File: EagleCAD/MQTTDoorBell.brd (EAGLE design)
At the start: 71.1 x 64.2 mm, 16 parts, among them Q1 MMBT2222

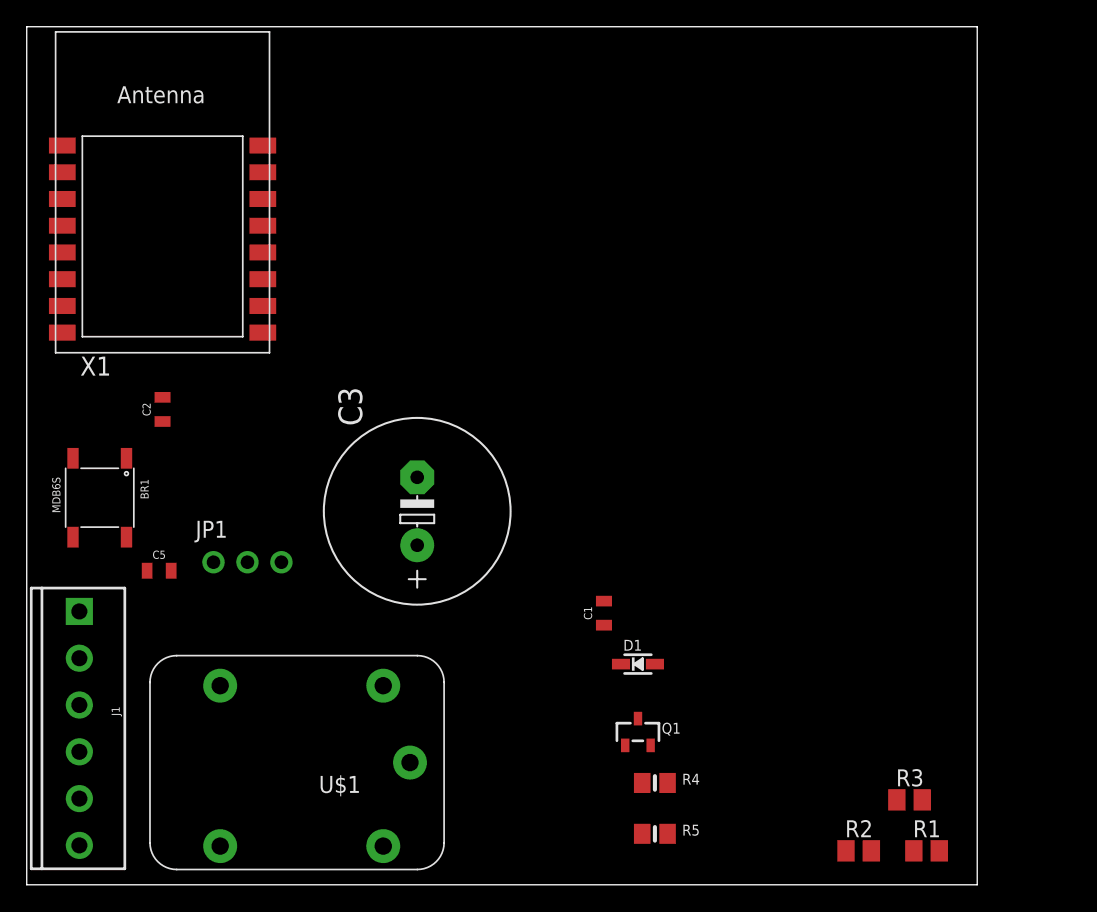
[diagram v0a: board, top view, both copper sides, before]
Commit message: initial commit of eagle files, version 1 of board'
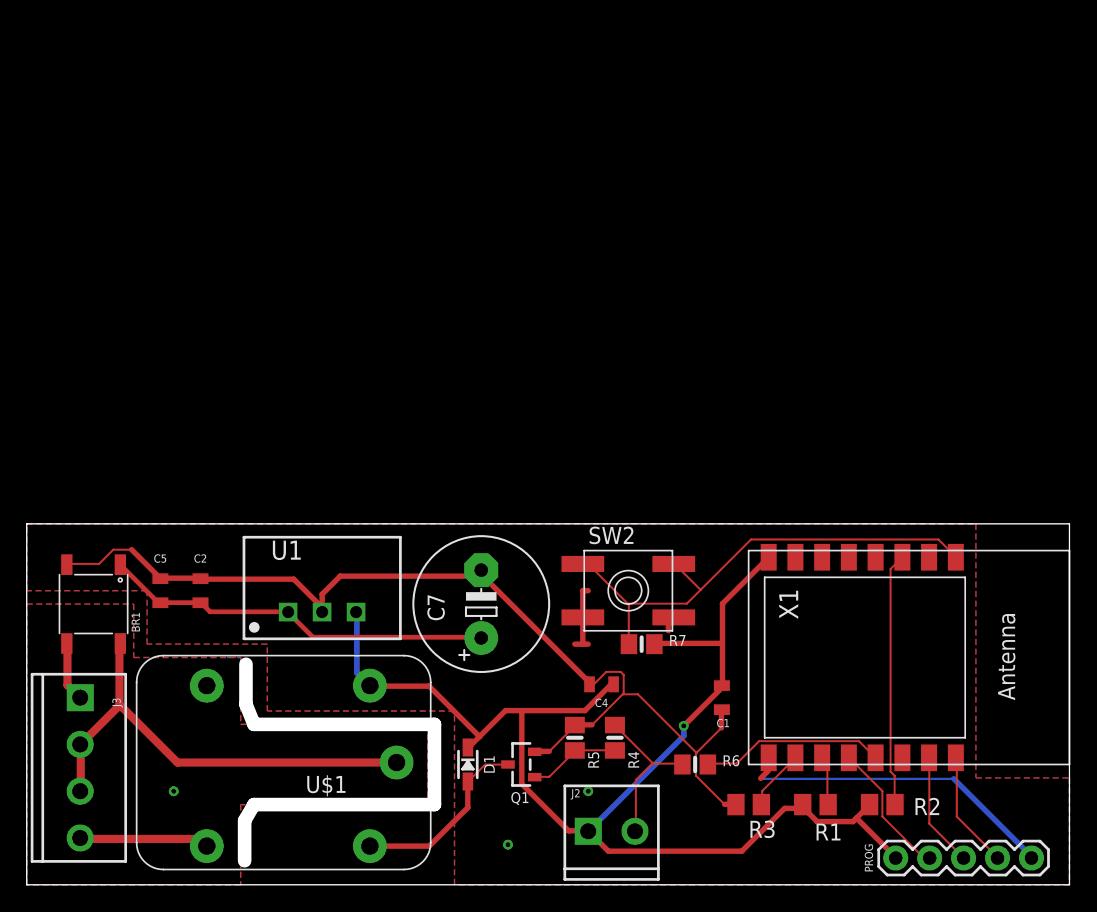
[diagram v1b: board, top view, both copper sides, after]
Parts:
- removed C3: (no value), adafruit:E5-13
- removed J1: (no value), SparkFun-Connectors:SCREWTERMINAL-3.5MM-6
- removed JP1: (no value), adafruit:1X03-CLEANBIG
- added C4: 10uf, SparkFun-Capacitors:0805
- added C7: (no value), adafruit:E5-10,5
- added J2: (no value), SparkFun-Connectors:SCREWTERMINAL-3.5MM-2
- added J3: (no value), SparkFun-Connectors:SCREWTERMINAL-3.5MM-4
- added PROG: (no value), SparkFun-Connectors:1X05
- added R6, R7: 2K, microbuilder:0805-NO
- added SW2: SPST_TACT-EVQQ2, adafruit:EVQ-Q2
- added U1: TSR_1-2433, Traco_TSR:TSR-1
- R1, R2, R3: value (none) -> 10k
- moved X1 64.4 mm to (65.0, 17.0), turned to 270 degrees
- moved D1 14.8 mm to (33.0, 9.00), turned to 270 degrees
- moved C2 13.9 mm to (13.0, 22.0)
- moved R3 12.0 mm to (54.0, 6.00)
- moved C1 10.9 mm to (52.0, 14.0), turned to 270 degrees
- moved R5 9.36 mm to (41.0, 11.0), turned to 270 degrees
- moved Q1 9.05 mm to (37.0, 9.00), turned to 90 degrees
- moved R1 9.00 mm to (59.0, 6.00), turned to 180 degrees
- moved BR1 7.97 mm to (5.00, 21.0)
- moved R4 4.51 mm to (44.0, 11.0), turned to 270 degrees
- moved R2 3.89 mm to (64.0, 6.00), turned to 180 degrees
- moved C5 1.50 mm to (10.0, 22.0), turned to 90 degrees
- moved U$1 1.00 mm to (19.3, 9.14)
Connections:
- removed net BUTTON2: J1.4
- new net GPIO0: PROG.2, X1.12
- new net RELAYDETECT: R6.2, X1.13
- new net RESET: R7.1, SW2.B, SW2.B', X1.1
- net 16V_AC1: now also J3.1; no longer J1.1, J1.5
- net 16V_AC2: now also J3.2, J3.3; no longer J1.2
- net 16V_DC: now also C7.+, U1.1; no longer C3.+, JP1.1
- net 3.3V: now also C4.1, J2.1, PROG.1, R7.2, U1.3; no longer JP1.3
- net BELL_OUT2: now also J3.4; no longer J1.6
- net BUTTON1: no longer J1.3
- net GND: now also C4.2, C7.-, PROG.5, SW2.A, SW2.A', U1.2; no longer C3.-, JP1.2
- net GPIO15: now also X1.10
- net GPIO2: now also X1.11
- net RELAYSIGNAL: now also J2.2, R6.1; no longer X1.12
- net RX: now also PROG.3
- net TX: now also PROG.4
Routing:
- net GND: track 0.00 -> 109.4 mm, vias 0 -> 2
- net 3.3V: track 0.00 -> 100.3 mm, vias 0 -> 1
- net RESET: track 0.00 -> 37.6 mm
- net 16V_AC2: track 0.00 -> 34.8 mm
- net 16V_DC: track 0.00 -> 29.3 mm
- net CH_PD: track 0.00 -> 19.0 mm
- net N$4: track 0.00 -> 14.0 mm
- net RELAYDETECT: track 0.00 -> 13.8 mm
- net RELAYSIGNAL: track 0.00 -> 11.9 mm
- net GPIO0: track 0.00 -> 10.3 mm
- net BELL_OUT2: track 0.00 -> 9.73 mm
- net TX: track 0.00 -> 8.80 mm
- net RX: track 0.00 -> 8.56 mm
- net N$22: track 0.00 -> 6.87 mm
- net GPIO15: track 0.00 -> 4.58 mm
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- added copper zone on layer 1, net ACISO1
- added copper zone on layer 16, net ACISO1
- added copper zone on layer 1, net GND
- added copper zone on layer 16, net GND
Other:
- board size 71.1 x 64.2 mm -> 78 x 27 mm
